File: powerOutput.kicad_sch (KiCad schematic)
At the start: 13 parts, among them IC14 LM5176PWPR, IC2 INA260AIPWR, IC3 INA260AIPWR, IC4 INA260AIPWR, IC5 TPS22990DMLR, IC6 TPS22990DMLR, IC7 TPS22990DMLR, Q1 BSZ067N06LS3_G, Q2 BSZ067N06LS3_G, Q3 BSZ067N06LS3_G

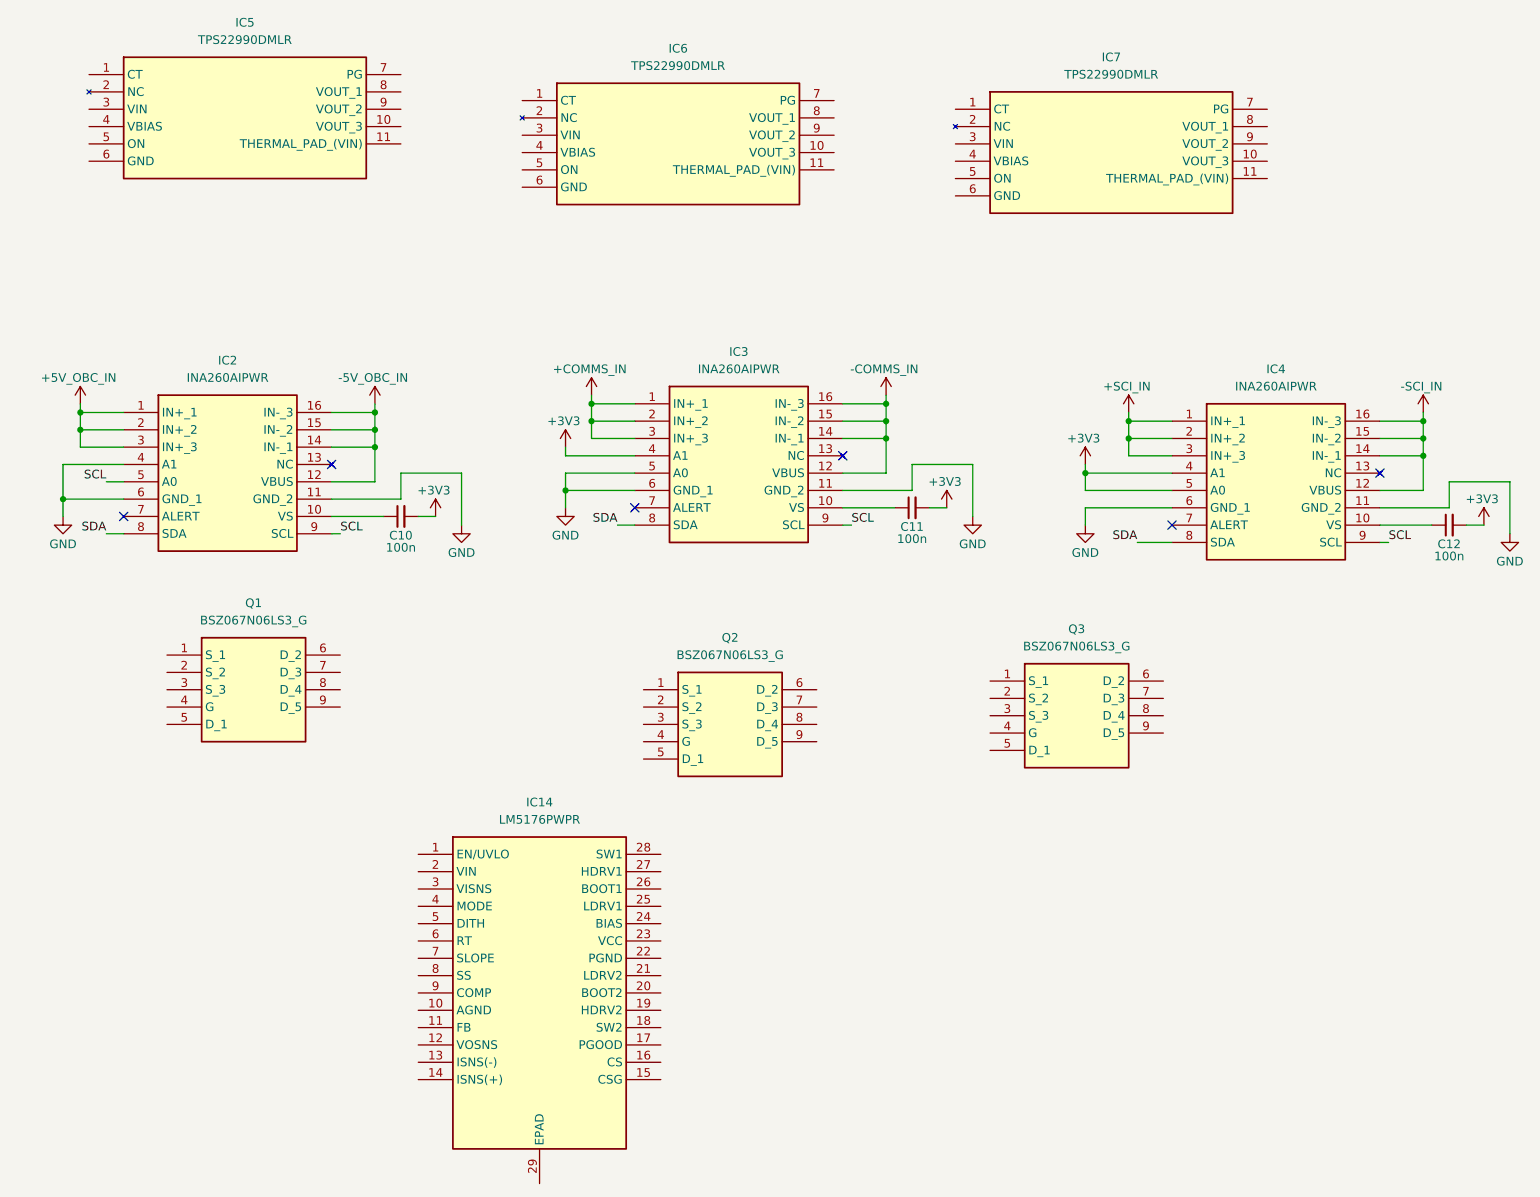
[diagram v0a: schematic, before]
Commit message: Test commit
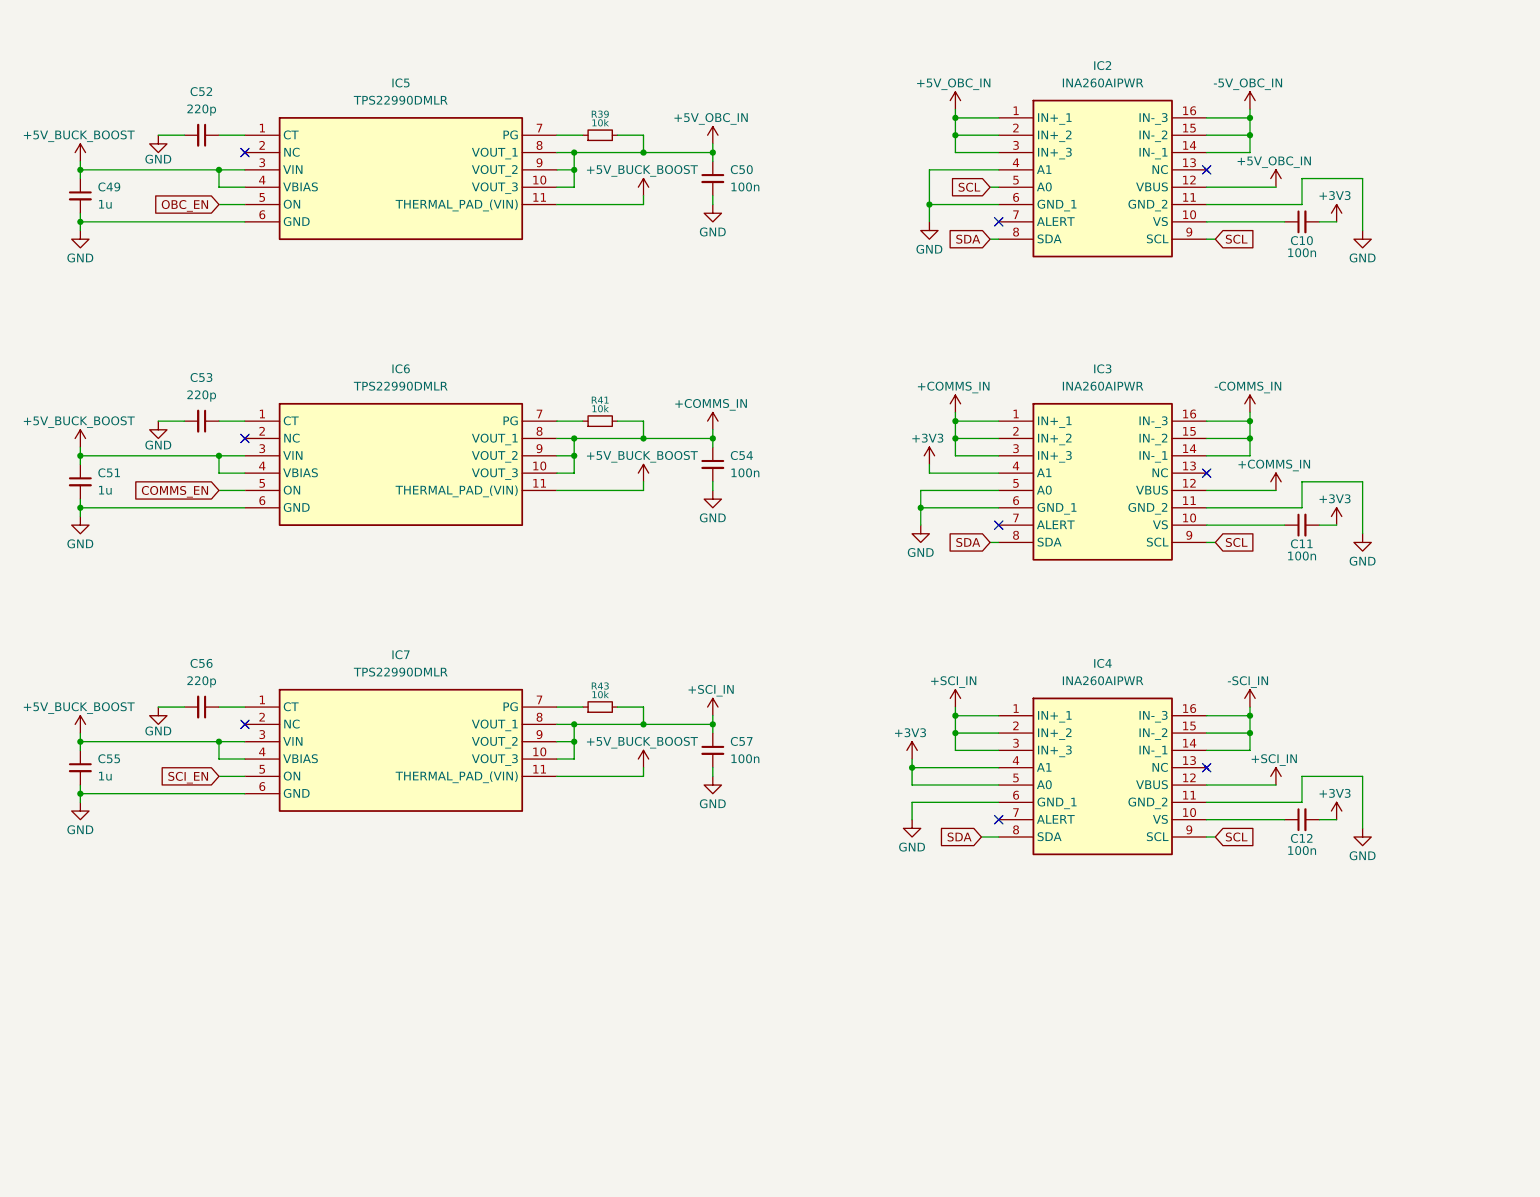
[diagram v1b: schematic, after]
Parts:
- removed IC14: LM5176PWPR, SOP65P640X120-29N, symbol HEDGE2:LM5176PWPR
- removed Q1, Q2, Q3: BSZ067N06LS3_G, BSZ067N06LS3G, symbol HEDGE2:BSZ067N06LS3_G
- added C49, C51, C55: 1u, symbol Device:C_Small
- added C50, C54, C57: 100n, symbol Device:C_Small
- added C52, C53, C56: 220p, symbol Device:C_Small
- added R39, R41, R43: 10k, symbol Device:R_Small
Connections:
- net +5V_OBC_IN: now also IC2.12 (VBUS), IC5.10 (VOUT_3), IC5.8 (VOUT_1), IC5.9 (VOUT_2), C50.1, R39.2
- net +COMMS_IN: now also IC3.12 (VBUS), IC6.10 (VOUT_3), IC6.8 (VOUT_1), IC6.9 (VOUT_2), C54.1, R41.2
- net +SCI_IN: now also IC4.12 (VBUS), IC7.10 (VOUT_3), IC7.8 (VOUT_1), IC7.9 (VOUT_2), C57.1, R43.2
- net -5V_OBC_IN: no longer IC2.12 (VBUS)
- net -COMMS_IN: no longer IC3.12 (VBUS)
- net -SCI_IN: no longer IC4.12 (VBUS)
- net GND: now also IC5.6 (GND), IC6.6 (GND), IC7.6 (GND), C49.2, C50.2, C51.2, C52.2, C53.2, C54.2, C55.2, C56.2, C57.2
- net at IC5.1 (CT): now also C52.1
- net +5V_BUCK_BOOST: now reaches IC5.11 (THERMAL_PAD_(VIN))
- net +5V_BUCK_BOOST: now also IC5.3 (VIN), IC5.4 (VBIAS), IC6.11 (THERMAL_PAD_(VIN)), IC6.3 (VIN), IC6.4 (VBIAS), IC7.11 (THERMAL_PAD_(VIN)), IC7.3 (VIN), IC7.4 (VBIAS), C49.1, C51.1, C55.1
- net OBC_EN: now reaches IC5.5 (ON)
- net at IC5.7 (PG): now also R39.1
- net at IC6.1 (CT): now also C53.1
- net COMMS_EN: now reaches IC6.5 (ON)
- net at IC6.7 (PG): now also R41.1
- net at IC7.1 (CT): now also C56.1
- net SCI_EN: now reaches IC7.5 (ON)
- net at IC7.7 (PG): now also R43.1
- no-connect marks 6 -> 9
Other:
- moved on the sheet: C10, C11, C12, IC2, IC3, IC4, IC5
